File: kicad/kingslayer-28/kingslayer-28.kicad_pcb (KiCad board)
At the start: 2 copper layers, 133 x 95 mm, 119 parts, among them IC1 STM32F303CCT7, IC2 IS31FL3731-QFLS2-TR, IC3 LM3940IMP-3.3_NOPB, J1 Conn_01x04_Pin, K1 KEYSW, K10 KEYSW, K11 KEYSW, K12 KEYSW, K13 KEYSW, K14 KEYSW, K15 KEYSW, K16 KEYSW, K17 KEYSW, K18 KEYSW, K19 KEYSW, K2 KEYSW, K20 KEYSW, K21 KEYSW, K22 KEYSW, K24 KEYSW, K25 KEYSW, K26 KEYSW, K27 KEYSW, K28 KEYSW, K3 KEYSW, K4 KEYSW, K5 KEYSW, K6 KEYSW, K7 KEYSW, K8 KEYSW, K9 KEYSW, SW1 SS12D07, X1 IC21008.000M30.0EE1B

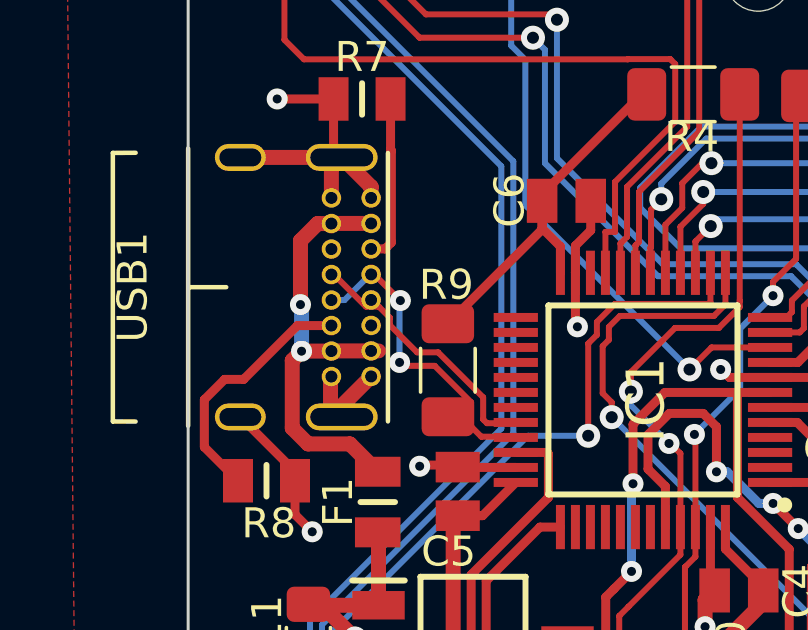
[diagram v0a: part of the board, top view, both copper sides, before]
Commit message: 3d model
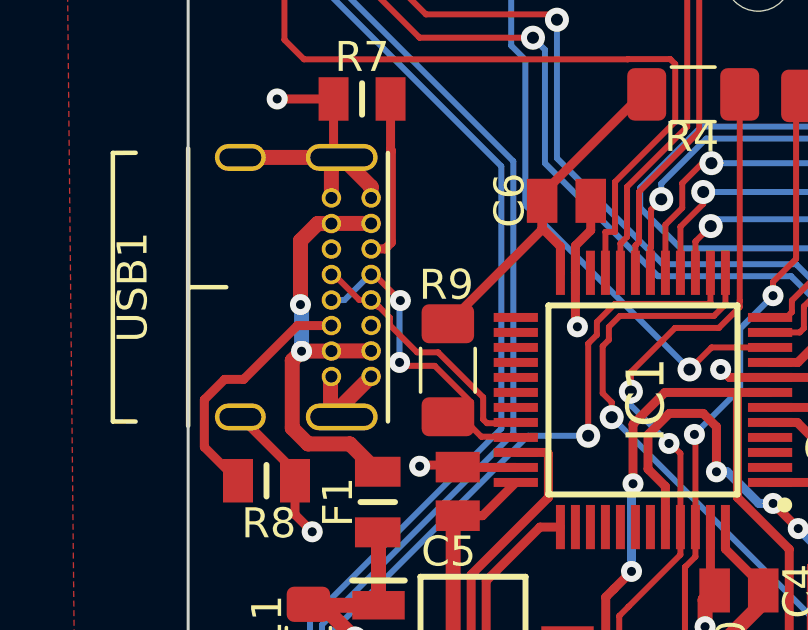
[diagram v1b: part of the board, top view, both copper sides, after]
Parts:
- USB1: footprint Type-C:USB_C_GCT_USB4085 -> custom:USB_C_GCT_USB4085
